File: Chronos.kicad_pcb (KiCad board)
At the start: 2 copper layers, 285 x 94.6 mm, 256 parts, among them Q1 NSS40301MZ4T1G, SW1 SW_PUSH, U1 ATMEGA32U2-AU, Y1 16MHz

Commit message: Change crystal
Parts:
- Y1: footprint Crystals:Crystal_SMD_3225-4pin_3.2x2.5mm_HandSoldering -> Crystals:Crystal_SMD_EuroQuartz_X22-4pin_2.5x2.0mm_HandSoldering
- moved R_RIGHT1 331.2 mm to (311.9, 138.1), turned to 270 degrees
- moved R_\1 328.6 mm to (329.8, 81.0), turned to 270 degrees
- moved R_RSHIFT1 326.9 mm to (315.5, 119.1), turned to 270 degrees
- moved R_DOWN1 319.4 mm to (298.8, 138.1), turned to 270 degrees
- moved R_BACK1 313.8 mm to (319.1, 61.9), turned to 270 degrees
- moved R_UP1 311.5 mm to (298.8, 119.1), turned to 270 degrees
- moved R_ENTER1 311.4 mm to (306.0, 100.0), turned to 270 degrees
- moved R_DEL1 304.5 mm to (309.6, 61.9), turned to 270 degrees
- moved R_/1 302.2 mm to (288.1, 120.3), turned to 180 degrees
- moved R_LEFT1 299.8 mm to (276.2, 139.3)
- moved R_ISO`1 297.2 mm to (290.5, 101.2)
- moved RGB14 291.2 mm to (231.0, 177.4)
- moved R_]1 289.6 mm to (289.3, 81.0), turned to 270 degrees
- moved RGB13 286.5 mm to (225.0, 177.4)
- moved R_`1 285.7 mm to (260.7, 138.1), turned to 270 degrees
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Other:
- net class POWER added: clearance 0.2, trace_width 0.381, via_dia 0.6, via_drill 0.4

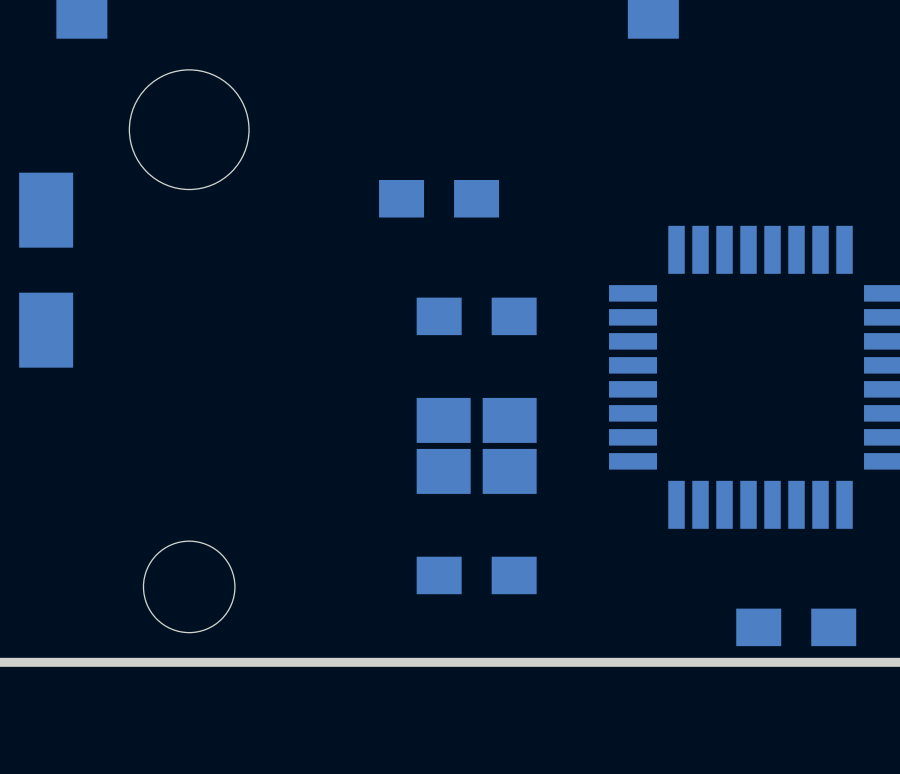
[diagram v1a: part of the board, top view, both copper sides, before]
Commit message: Change crystal back
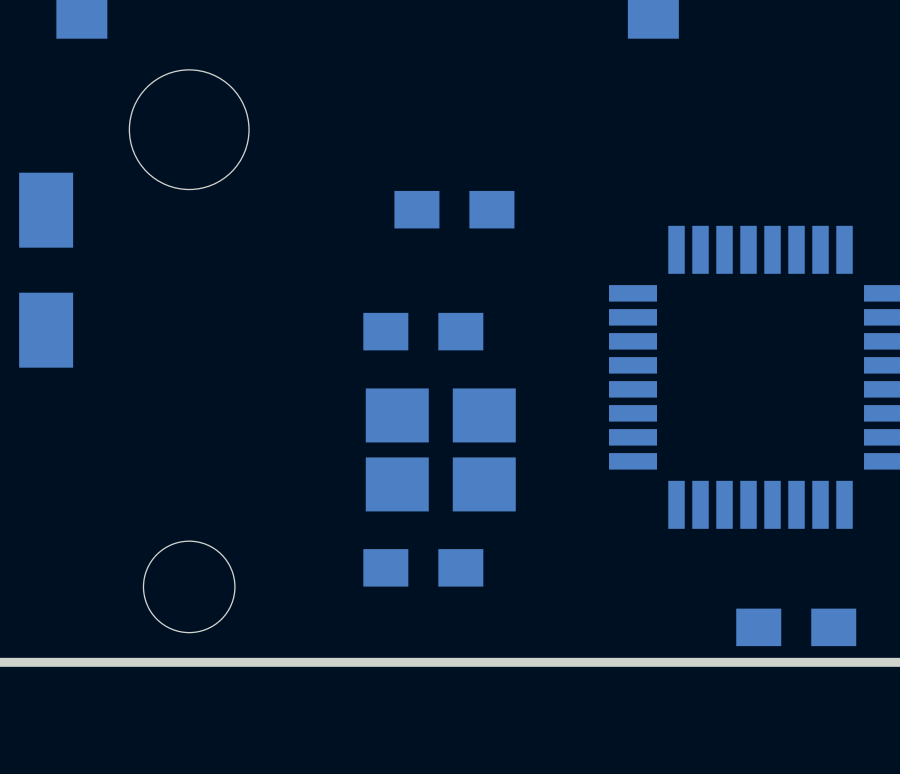
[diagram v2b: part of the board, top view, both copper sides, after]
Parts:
- Y1: footprint Crystals:Crystal_SMD_EuroQuartz_X22-4pin_2.5x2.0mm_HandSoldering -> Crystals:Crystal_SMD_3225-4pin_3.2x2.5mm_HandSoldering
- moved C2 1.85 mm to (136.4, 131.8)
- moved C1 1.80 mm to (136.4, 139.7)
- moved Y1 1.20 mm to (137.0, 135.8)
- moved C4 0.63 mm to (137.4, 127.8)
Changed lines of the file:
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@@
   (general
     (links 641)
-    (no_connects 451)
+    (no_connects 448)
     (area 0 0 0 0)
     (thickness 1.6)
@@
   )
   (module Capacitors_SMD:C_0805_HandSoldering (layer B.Cu)
-    (at 138.176 139.954 180)
+    (at 136.398 139.7 180)
     (descr "Capacitor SMD 0805, hand soldering")
     (tags "capacitor 0805")
@@
   )
   (module Capacitors_SMD:C_0805_HandSoldering (layer B.Cu)
-    (at 138.176 131.318)
+    (at 136.398 131.826)
     (descr "Capacitor SMD 0805, hand soldering")
     (tags "capacitor 0805")
@@
   )
   (module Capacitors_SMD:C_0805_HandSoldering (layer B.Cu)
-    (at 136.921875 127.396875 180)
+    (at 137.434 127.762 180)
     (descr "Capacitor SMD 0805, hand soldering")
     (tags "capacitor 0805")
@@
     (pad "" np_thru_hole circle (at 5.08 0 48.0996) (size 1.7018 1.7018) (drill 1.7018) (layers *.Cu *.Mask))
   )
-  (module Crystals:Crystal_SMD_EuroQuartz_X22-4pin_2.5x2.0mm_HandSoldering (layer B.Cu)
-    (at 138.176 135.636 180)
-    (descr "SMD Crystal EuroQuartz X22 series http://cdn-reichelt.de/documents/datenblatt/B400/DS_X22.pdf, hand-soldering, 2.5x2.0mm^2 package")
+  (module Crystals:Crystal_SMD_3225-4pin_3.2x2.5mm_HandSoldering (layer B.Cu)
+    (at 136.98 135.77 180)
+    (descr "SMD Crystal SERIES SMD3225/4 http://www.txccrystal.com/images/pdf/7m-accuracy.pdf, hand-soldering, 3.2x2.5mm^2 package")
     (tags "SMD SMT crystal hand-soldering")
     (attr smd)
-    (fp_text reference Y1 (at 0 2.6 180) (layer B.SilkS)
+    (fp_text reference Y1 (at 0 3.05 180) (layer B.SilkS)
       (effects (font (size 1 1) (thickness 0.15)) (justify mirror))
     )
-    (fp_text value 16MHz (at 0 -2.6 180) (layer B.Fab)
+    (fp_text value 16MHz (at 0 -3.05 180) (layer B.Fab)
       (effects (font (size 1 1) (thickness 0.15)) (justify mirror))
     )
     (fp_text user %R (at 0 0 180) (layer B.Fab)
-      (effects (font (size 0.6 0.6) (thickness 0.09)) (justify mirror))
+      (effects (font (size 0.7 0.7) (thickness 0.105)) (justify mirror))
     )
-    (fp_line (start -1.15 1) (end 1.15 1) (layer B.Fab) (width 0.1))
-    (fp_line (start 1.15 1) (end 1.25 0.9) (layer B.Fab) (width 0.1))
-    (fp_line (start 1.25 0.9) (end 1.25 -0.9) (layer B.Fab) (width 0.1))
-    (fp_line (start 1.25 -0.9) (end 1.15 -1) (layer B.Fab) (width 0.1))
-    (fp_line (start 1.15 -1) (end -1.15 -1) (layer B.Fab) (width 0.1))
-    (fp_line (start -1.15 -1) (end -1.25 -0.9) (layer B.Fab) (width 0.1))
-    (fp_line (start -1.25 -0.9) (end -1.25 0.9) (layer B.Fab) (width 0.1))
-    (fp_line (start -1.25 0.9) (end -1.15 1) (layer B.Fab) (width 0.1))
-    (fp_line (start -1.25 0) (end -0.25 -1) (layer B.Fab) (width 0.1))
-    (fp_line (start -2.2 1.8) (end -2.2 -1.8) (layer B.SilkS) (width 0.12))
-    (fp_line (start -2.2 -1.8) (end 2.2 -1.8) (layer B.SilkS) (width 0.12))
-    (fp_line (start -2.3 1.9) (end -2.3 -1.9) (layer B.CrtYd) (width 0.05))
-    (fp_line (start -2.3 -1.9) (end 2.3 -1.9) (layer B.CrtYd) (width 0.05))
-    (fp_line (start 2.3 -1.9) (end 2.3 1.9) (layer B.CrtYd) (width 0.05))
-    (fp_line (start 2.3 1.9) (end -2.3 1.9) (layer B.CrtYd) (width 0.05))
-    (pad 1 smd rect (at -1.1 -0.85 180) (size 1.8 1.5) (layers B.Cu B.Paste B.Mask)
+    (fp_line (start -1.6 1.25) (end -1.6 -1.25) (layer B.Fab) (width 0.1))
+    (fp_line (start -1.6 -1.25) (end 1.6 -1.25) (layer B.Fab) (width 0.1))
+    (fp_line (start 1.6 -1.25) (end 1.6 1.25) (layer B.Fab) (width 0.1))
+    (fp_line (start 1.6 1.25) (end -1.6 1.25) (layer B.Fab) (width 0.1))
+    (fp_line (start -1.6 -0.25) (end -0.6 -1.25) (layer B.Fab) (width 0.1))
+    (fp_line (start -2.7 2.25) (end -2.7 -2.25) (layer B.SilkS) (width 0.12))
+    (fp_line (start -2.7 -2.25) (end 2.7 -2.25) (layer B.SilkS) (width 0.12))
+    (fp_line (start -2.8 2.3) (end -2.8 -2.3) (layer B.CrtYd) (width 0.05))
+    (fp_line (start -2.8 -2.3) (end 2.8 -2.3) (layer B.CrtYd) (width 0.05))
+    (fp_line (start 2.8 -2.3) (end 2.8 2.3) (layer B.CrtYd) (width 0.05))
+    (fp_line (start 2.8 2.3) (end -2.8 2.3) (layer B.CrtYd) (width 0.05))
+    (pad 1 smd rect (at -1.45 -1.15 180) (size 2.1 1.8) (layers B.Cu B.Paste B.Mask)
       (net 1 "Net-(C1-Pad1)"))
-    (pad 2 smd rect (at 1.1 -0.85 180) (size 1.8 1.5) (layers B.Cu B.Paste B.Mask)
+    (pad 2 smd rect (at 1.45 -1.15 180) (size 2.1 1.8) (layers B.Cu B.Paste B.Mask)
       (net 2 GND))
-    (pad 3 smd rect (at 1.1 0.85 180) (size 1.8 1.5) (layers B.Cu B.Paste B.Mask)
+    (pad 3 smd rect (at 1.45 1.15 180) (size 2.1 1.8) (layers B.Cu B.Paste B.Mask)
       (net 3 "Net-(C2-Pad1)"))
-    (pad 4 smd rect (at -1.1 0.85 180) (size 1.8 1.5) (layers B.Cu B.Paste B.Mask)
+    (pad 4 smd rect (at -1.45 1.15 180) (size 2.1 1.8) (layers B.Cu B.Paste B.Mask)
       (net 2 GND))
-    (model ${KISYS3DMOD}/Crystals.3dshapes/Crystal_SMD_EuroQuartz_X22-4pin_2.5x2.0mm_HandSoldering.wrl
+    (model ${KISYS3DMOD}/Crystals.3dshapes/Crystal_SMD_3225-4pin_3.2x2.5mm_HandSoldering.wrl
       (at (xyz 0 0 0))
       (scale (xyz 1 1 1))
